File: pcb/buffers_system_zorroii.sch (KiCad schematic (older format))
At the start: 37 parts, among them U5 74LVCH162245A

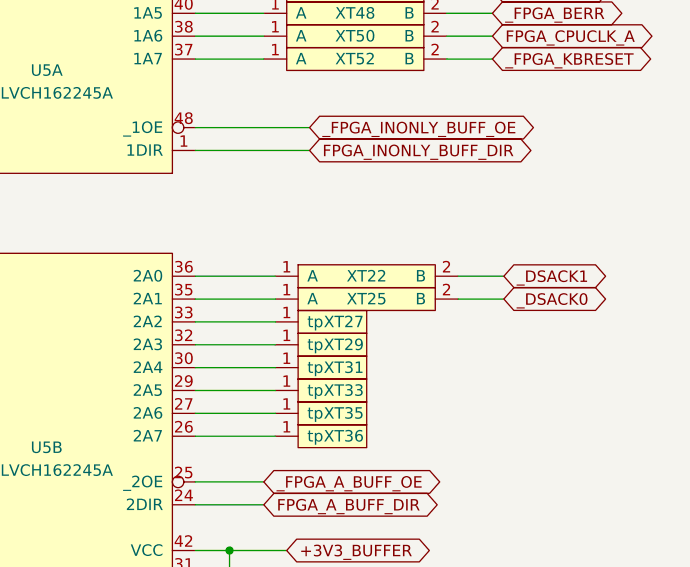
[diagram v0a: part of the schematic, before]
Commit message: some work on hdmi part
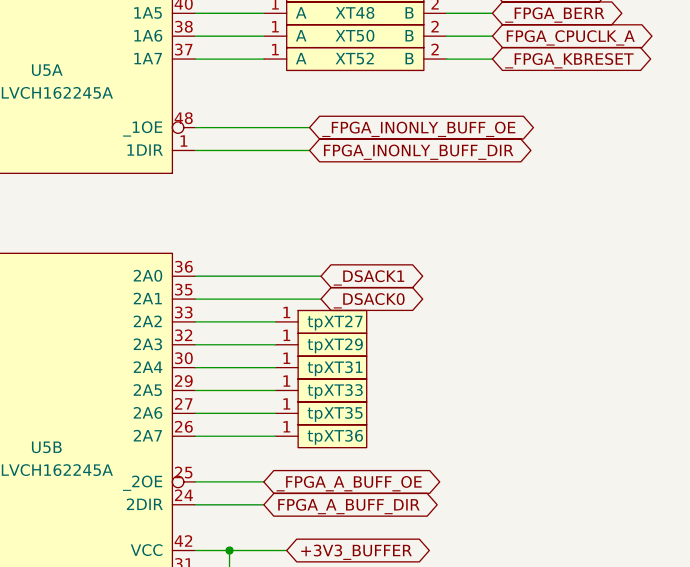
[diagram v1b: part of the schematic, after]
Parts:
- removed XT22, XT25: testpoint_cutline, WM1200:testpoint_cutline, symbol WM1200:testpoint_cutline
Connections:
- net _DSACK0: now also U5.35 (2A1)
- net _DSACK1: now also U5.36 (2A0)
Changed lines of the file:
@@
 	3150 2250 3500 2250
-$Comp
-L WM1200:testpoint_cutline XT22
-U 1 1 5E96BD33
-P 5550 3250
-F 0 "XT22" H 5550 3300 50  0000 C CNN
-F 1 "testpoint_cutline" H 5550 3400 50  0001 C CNN
-F 2 "WM1200:testpoint_cutline" H 5700 3250 50  0001 C CNN
-F 3 "" H 5700 3250 50  0001 C CNN
-	1    5550 3250
-	1    0    0    -1
-$EndComp
 $Comp
 L WM1200:testpoint XT27
@@
 F 3 "" H 5400 3450 50  0001 C CNN
 	1    5400 3450
-	1    0    0    -1
-$EndComp
-$Comp
-L WM1200:testpoint_cutline XT25
-U 1 1 5E96CD4A
-P 5550 3350
-F 0 "XT25" H 5550 3400 50  0000 C CNN
-F 1 "testpoint_cutline" H 5550 3500 50  0001 C CNN
-F 2 "WM1200:testpoint_cutline" H 5700 3350 50  0001 C CNN
-F 3 "" H 5700 3350 50  0001 C CNN
-	1    5550 3350
 	1    0    0    -1
 $EndComp
@@
 $EndComp
 Wire Wire Line
-	5150 3200 4800 3200
-Wire Wire Line
-	4800 3300 5150 3300
-Wire Wire Line
 	5150 3400 4800 3400
 Wire Wire Line
@@
 Wire Wire Line
 	4800 3900 5150 3900
-Wire Wire Line
-	5950 3200 6150 3200
-Wire Wire Line
-	6150 3300 5950 3300
-Text GLabel 6150 3300 2    50   BiDi ~ 0
+Text GLabel 5350 3300 2    50   BiDi ~ 0
 _DSACK0
-Text GLabel 6150 3200 2    50   BiDi ~ 0
+Text GLabel 5350 3200 2    50   BiDi ~ 0
 _DSACK1
 Wire Wire Line
@@
 Wire Wire Line
 	4800 2650 5300 2650
+Wire Wire Line
+	4800 3200 5350 3200
+Wire Wire Line
+	4800 3300 5350 3300
 $EndSCHEMATC

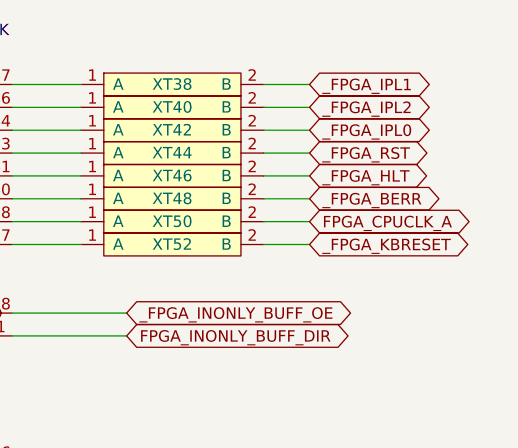
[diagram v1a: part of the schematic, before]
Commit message: some more work done
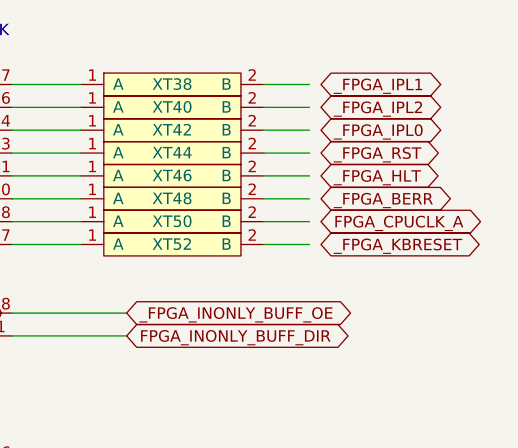
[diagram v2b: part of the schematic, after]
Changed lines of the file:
@@
 	5200 4400 4950 4400
 Connection ~ 4950 4400
-Text GLabel 6100 2050 2    50   BiDi ~ 0
+Text GLabel 6150 2050 2    50   BiDi ~ 0
 _FPGA_BERR
-Text GLabel 6100 2150 2    50   BiDi ~ 0
+Text GLabel 6150 2150 2    50   BiDi ~ 0
 FPGA_CPUCLK_A
-Text GLabel 6100 1950 2    50   BiDi ~ 0
+Text GLabel 6150 1950 2    50   BiDi ~ 0
 _FPGA_HLT
-Text GLabel 6100 1650 2    50   BiDi ~ 0
+Text GLabel 6150 1650 2    50   BiDi ~ 0
 _FPGA_IPL2
-Text GLabel 6100 1550 2    50   BiDi ~ 0
+Text GLabel 6150 1550 2    50   BiDi ~ 0
 _FPGA_IPL1
-Text GLabel 6100 1750 2    50   BiDi ~ 0
+Text GLabel 6150 1750 2    50   BiDi ~ 0
 _FPGA_IPL0
-Text GLabel 6100 1850 2    50   BiDi ~ 0
+Text GLabel 6150 1850 2    50   BiDi ~ 0
 _FPGA_RST
-Text GLabel 6100 2250 2    50   BiDi ~ 0
+Text GLabel 6150 2250 2    50   BiDi ~ 0
 _FPGA_KBRESET
 Text GLabel 5300 2550 2    50   BiDi ~ 0
